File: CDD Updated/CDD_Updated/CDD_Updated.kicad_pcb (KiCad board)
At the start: 4 copper layers, 34.8 x 29 mm, 6 parts, among them J1 B2B-XH-A, U1 DPS368XTSA1_PRESSURE_SENSOR, U2 MAX30101, U3 MOUDLE-SEEEDUINO-XIAO-ESP32C3

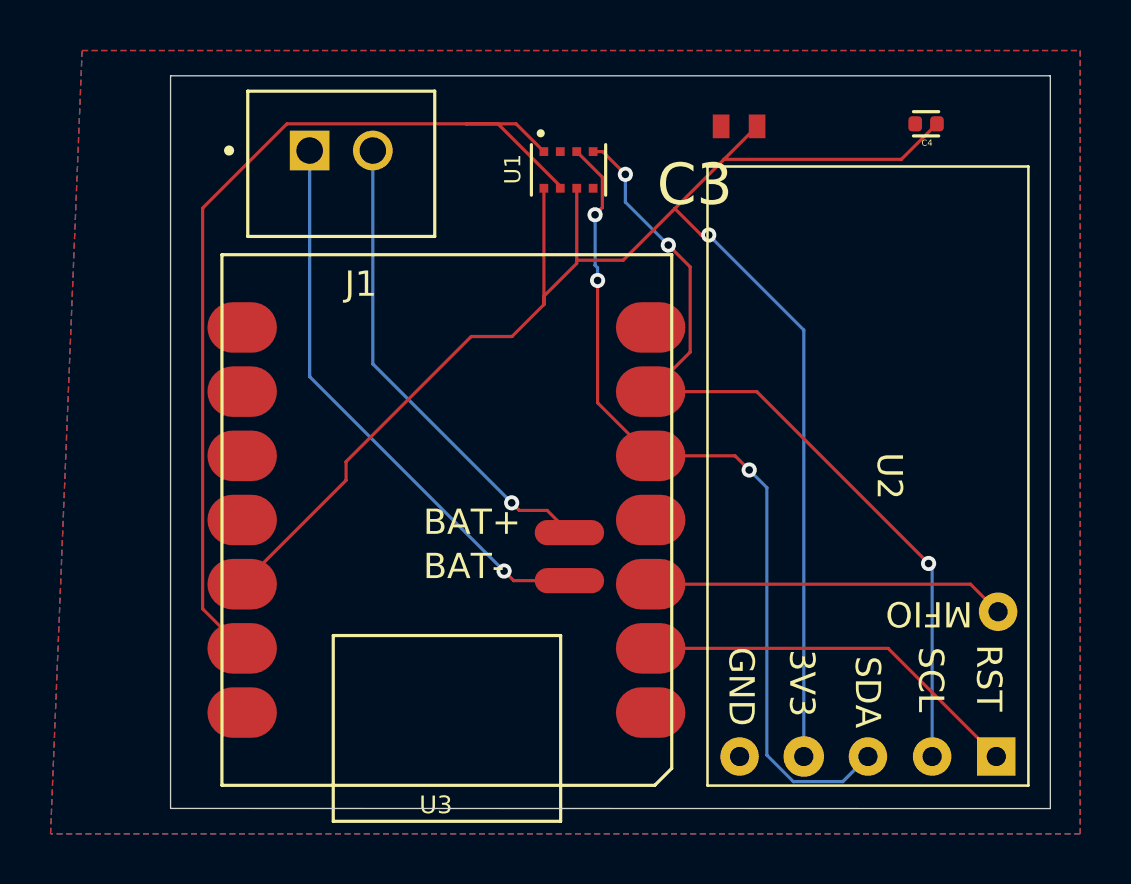
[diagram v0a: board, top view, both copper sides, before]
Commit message: Update PCB
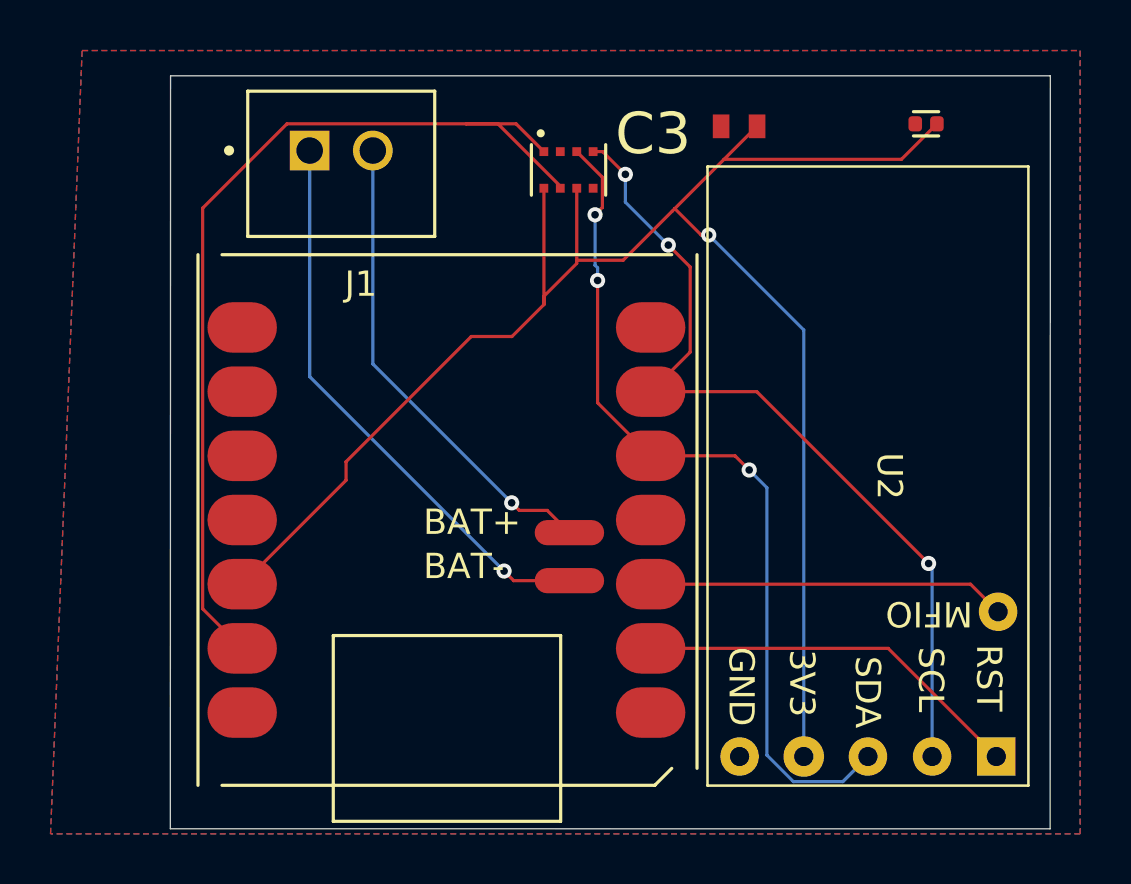
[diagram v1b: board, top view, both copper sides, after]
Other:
- board size 34.8 x 29 mm -> 34.8 x 29.8 mm
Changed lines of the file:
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@@
 		(at 127 79 180)
 		(property "Reference" "C3"
-			(at 1.7526 -2.3114 360)
+			(at 3.4 -0.3 0)
 			(layer "F.SilkS")
 			(effects
@@
 			(at 9.0424 2.1336 90)
 			(layer "F.Fab")
+			(hide yes)
 			(effects
 				(font
@@
 		)
 		(property "Footprint" "CDD Updated:CAPC1608X90N_47uF"
-			(at 0 0 360)
+			(at 0 0 0)
 			(layer "F.Fab")
 			(hide yes)
@@
 		)
 		(property "Datasheet" ""
-			(at 0 0 360)
+			(at 0 0 0)
 			(layer "F.Fab")
 			(hide yes)
@@
 		)
 		(property "Description" ""
-			(at 0 0 360)
+			(at 0 0 0)
 			(layer "F.Fab")
 			(hide yes)
@@
 		(at 111.2552 80.4826 180)
 		(property "Reference" "J1"
-			(at -0.775 -4.76 360)
+			(at -0.775 -4.76 0)
 			(layer "F.SilkS")
 			(effects
@@
 		)
 		(property "Value" "B2B-XH-A"
-			(at 3.67 4.76 360)
-			(layer "F.Fab")
+			(at 3.67 4.76 0)
+			(layer "F.Fab")
+			(hide yes)
 			(effects
 				(font
@@
 		)
 		(property "Footprint" "CDD Updated:JST_B2B-XH-A"
-			(at 0 0 360)
+			(at 0 0 0)
 			(layer "F.Fab")
 			(hide yes)
@@
 		)
 		(property "Datasheet" ""
-			(at 0 0 360)
+			(at 0 0 0)
 			(layer "F.Fab")
 			(hide yes)
@@
 		)
 		(property "Description" ""
-			(at 0 0 360)
+			(at 0 0 0)
 			(layer "F.Fab")
 			(hide yes)
@@
 			(at 9.3345 -21.7805 0)
 			(layer "F.SilkS")
+			(hide yes)
 			(effects
 				(font
@@
 		(attr through_hole)
 		(fp_line
-			(start 17.8 0)
-			(end 17.8 -21)
+			(start 18.75 0)
+			(end 18.75 -21)
 			(stroke
 				(width 0.127)
@@
 		)
 		(fp_line
-			(start 0 -20.3285)
-			(end 0 0)
+			(start -1 -20.3285)
+			(end -1 0)
 			(stroke
 				(width 0.127)
@@
 			(at 0.032 -2.2064 90)
 			(layer "F.SilkS")
+			(hide yes)
 			(effects
 				(font
@@
 		(sheetname "Root")
 		(sheetfile "CDD_Updated.kicad_sch")
-		(attr smd)
+		(attr smd allow_soldermask_bridges)
 		(fp_circle
 			(center 0.725 -0.975)
@@
 		(at 134.4 78.9 180)
 		(property "Reference" "C4"
-			(at -0.038171 -0.755633 360)
-			(layer "F.SilkS")
+			(at -0.038171 -0.755633 0)
+			(layer "F.SilkS")
+			(hide yes)
 			(effects
 				(font
 					(size 0.241029 0.241029)
-					(thickness 0.15)
+					(thickness 0.060257)
 				)
 			)
 		)
 		(property "Value" "CL05B104KP5NNNC"
-			(at 1.032975 0.851042 360)
-			(layer "F.Fab")
+			(at 1.032975 0.851042 0)
+			(layer "F.Fab")
+			(hide yes)
 			(effects
 				(font
 					(size 0.240973 0.240973)
-					(thickness 0.15)
+					(thickness 0.060243)
 				)
 			)
 		)
 		(property "Footprint" "CDD Updated:CAPC1005X55N_0.1NF"
-			(at 0 0 360)
+			(at 0 0 0)
 			(layer "F.Fab")
 			(hide yes)
@@
 		)
 		(property "Datasheet" ""
-			(at 0 0 360)
+			(at 0 0 0)
 			(layer "F.Fab")
 			(hide yes)
@@
 		)
 		(property "Description" ""
-			(at 0 0 360)
+			(at 0 0 0)
 			(layer "F.Fab")
 			(hide yes)
@@
 		(sheetname "Root")
 		(sheetfile "CDD_Updated.kicad_sch")
-		(attr smd)
+		(attr smd allow_soldermask_bridges)
 		(fp_line
 			(start 0.5 -0.48)
@@
 	(gr_line
 		(start 104.5 77)
-		(end 104.5 105.995)
+		(end 104.4905 106.7975)
 		(stroke
 			(width 0.0381)
@@
 	)
 	(gr_line
-		(start 139.319 106)
+		(start 139.3095 106.8025)
 		(end 139.319 77)
 		(stroke
@@
 	)
 	(gr_line
-		(start 104.5 105.995)
-		(end 139.319 106)
+		(start 104.4905 106.7975)
+		(end 139.3095 106.8025)
 		(stroke
 			(width 0.0381)
